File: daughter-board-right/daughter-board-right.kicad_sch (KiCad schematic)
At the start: 20 parts, among them J1 Conn_01x06_MountingPin, J2 USB_C_Receptacle_USB2.0_16P, J3 PJ-320A, U1 SRV05-4

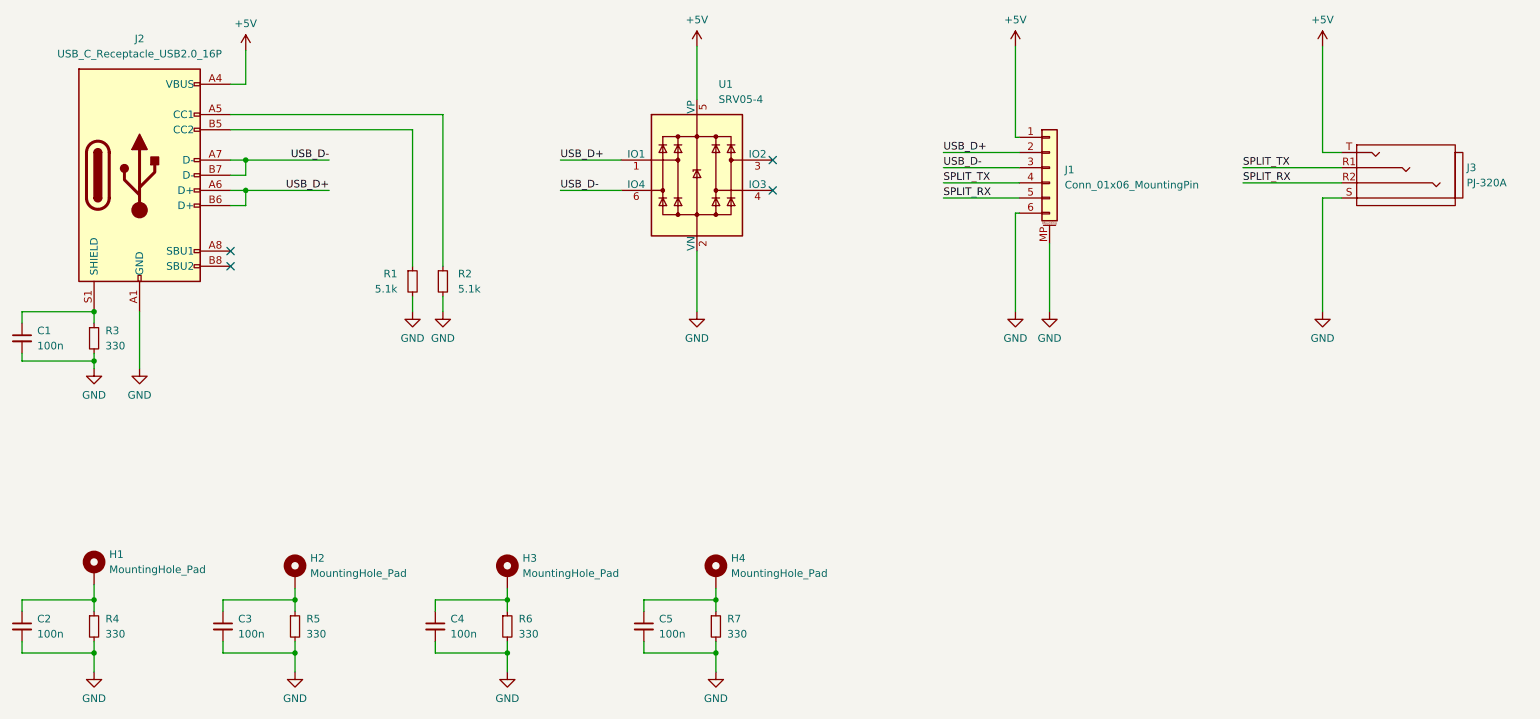
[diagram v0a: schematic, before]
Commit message: quick save
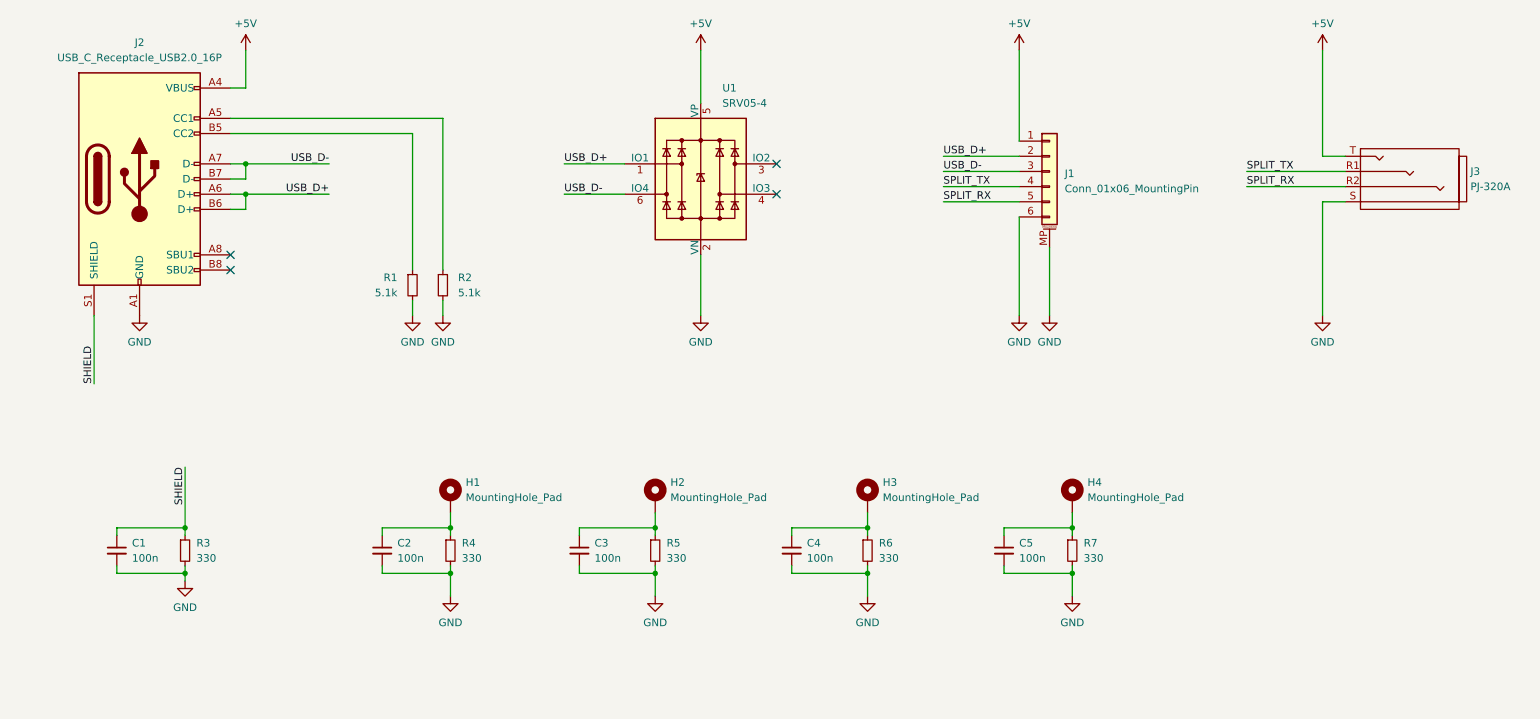
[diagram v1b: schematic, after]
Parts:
- J1: footprint Connector_JST:JST_SHL_SM06B-SHLS-TF_1x06-1MP_P1.00mm_Horizontal -> Connector_JST:JST_SH_SM06B-SRSS-TB_1x06-1MP_P1.00mm_Horizontal
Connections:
- net SHIELD: now reaches C1.1, J2.S1 (SHIELD), R3.1
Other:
- moved on the sheet: C1, C2, C3, C4, C5, H1, H2, H3, H4, J1, J2, J3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
